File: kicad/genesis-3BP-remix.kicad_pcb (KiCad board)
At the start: 2 copper layers, 29 x 38.5 mm, 91 parts, among them CON1 MD-90SM, J1 S, J10 XL, J11 CL, J12 YL, J2 R, J3 G, J4 B, J5 VS, J6 YR, J7 CR, J8 XR, J9 PSG, M1PU1 Jumper, U1 THS7374, U2 TLV9062xD

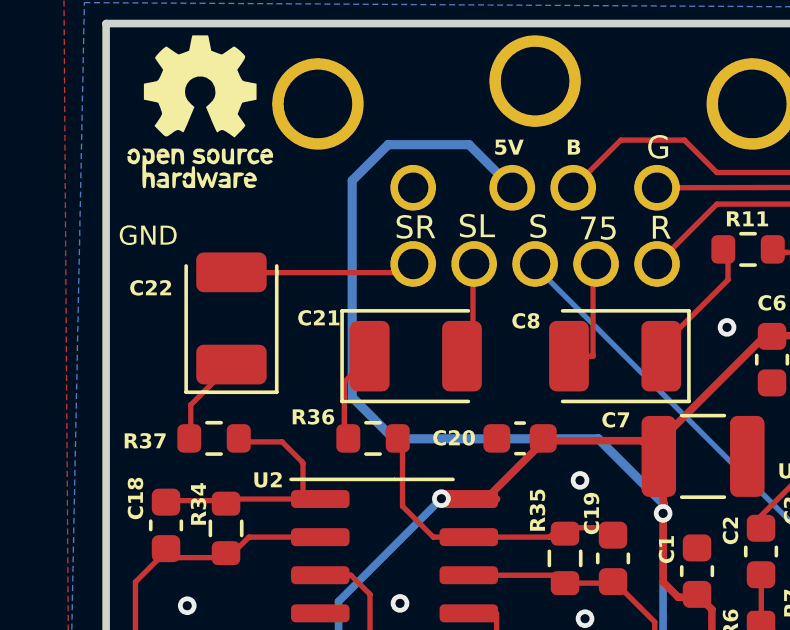
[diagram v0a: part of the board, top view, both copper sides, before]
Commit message: Update cap pad change
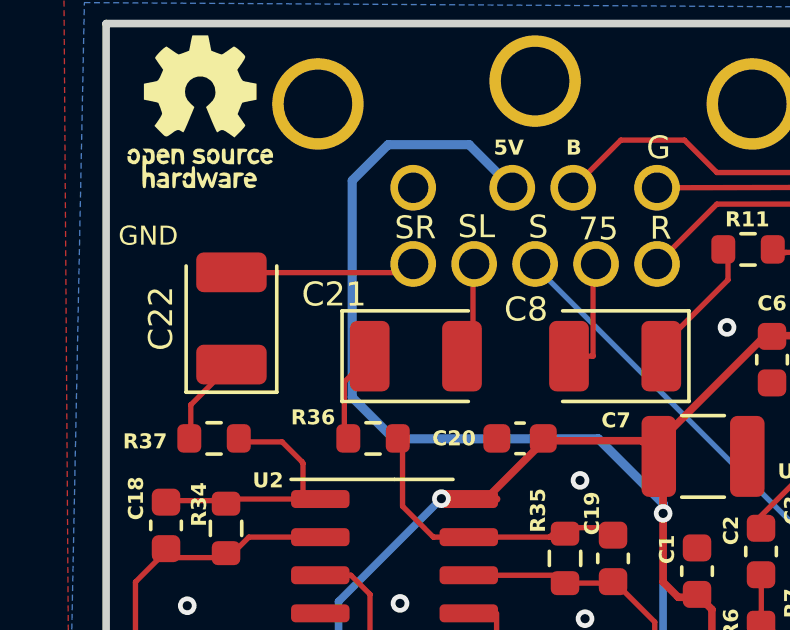
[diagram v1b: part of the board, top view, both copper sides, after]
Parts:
- C21, C22, C8: footprint Capacitor_Tantalum_SMD:CP_EIA-3528-21_Kemet-B -> Capacitor_Tantalum_SMD:CP_EIA-3528-15_AVX-H
